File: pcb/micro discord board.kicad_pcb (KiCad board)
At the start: 2 copper layers, 71.4 x 57.2 mm, 9 parts, among them SW1 SW_Push, SW2 SW_Push, SW3 SW_Push, SW4 SW_Push, SW5 RotaryEncoder, U1 XIAO-RP2040-DIP

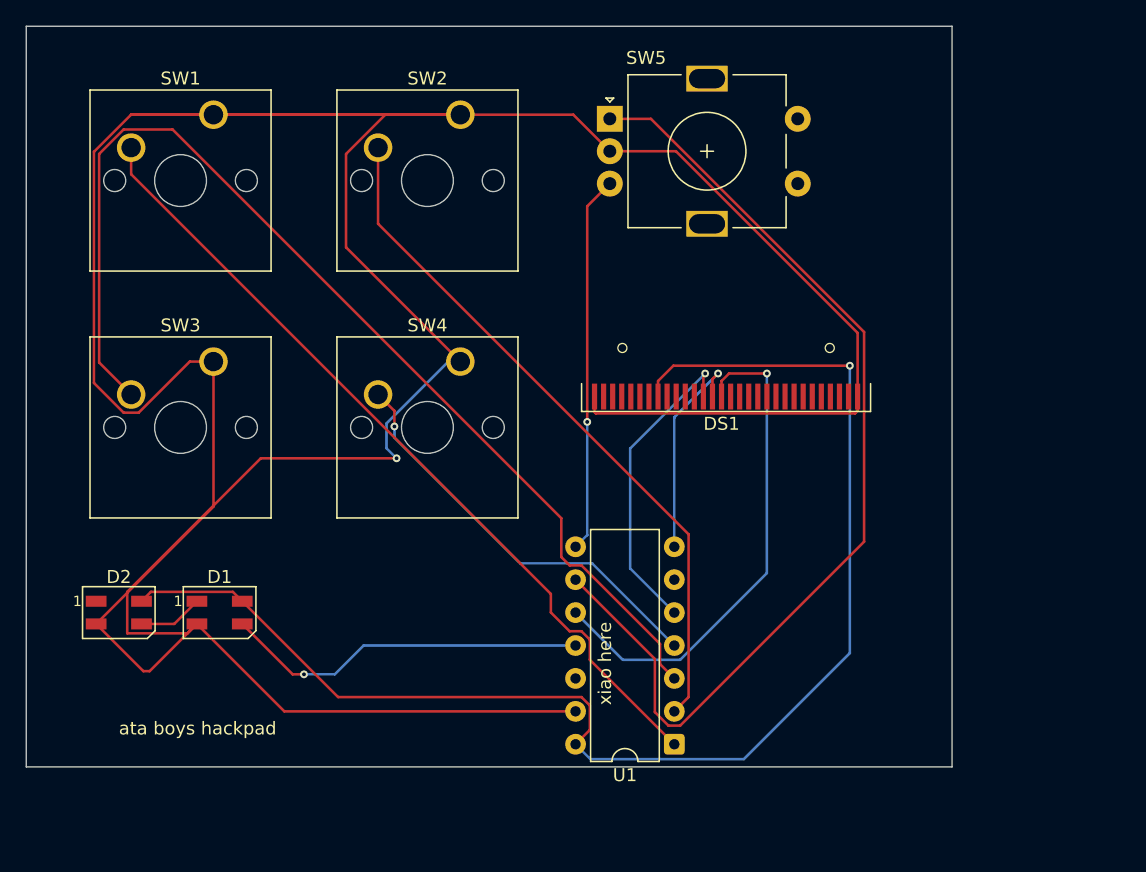
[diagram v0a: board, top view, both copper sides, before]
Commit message: Add files via upload
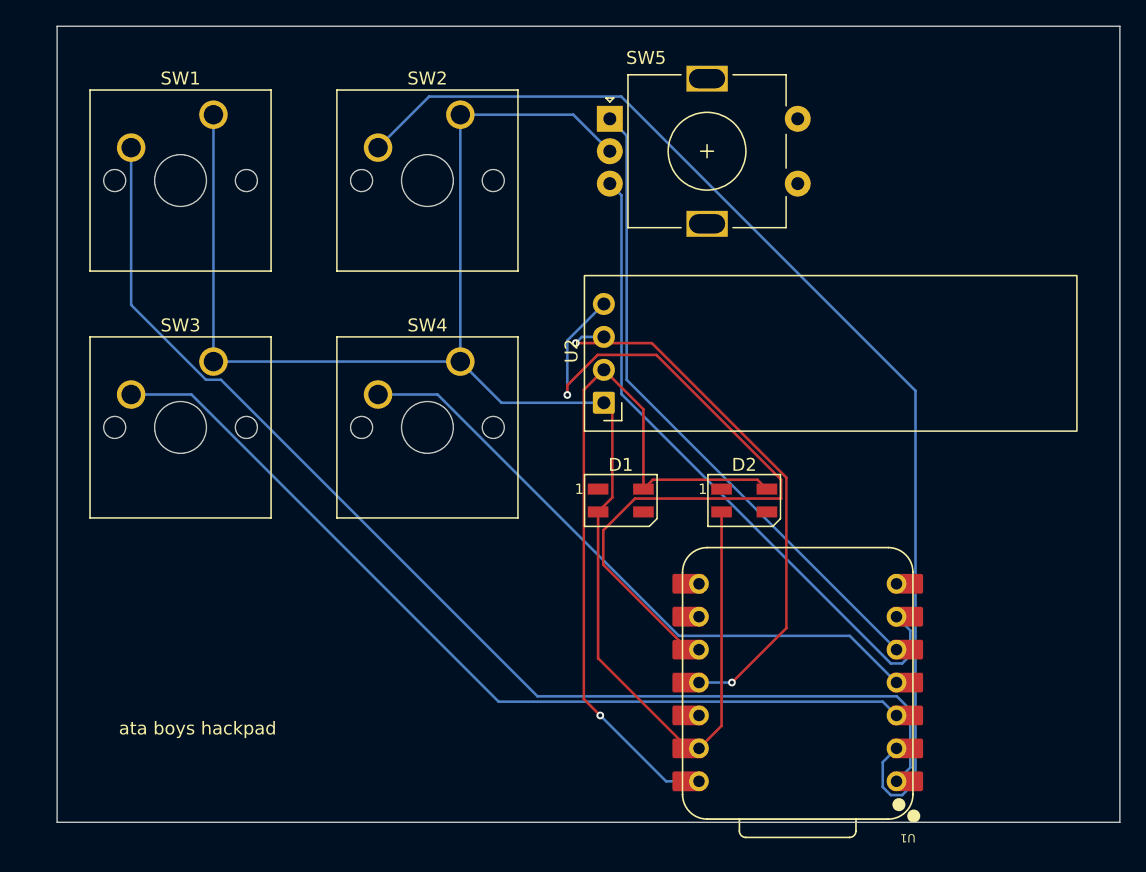
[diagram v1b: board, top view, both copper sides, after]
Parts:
- removed DS1: OLED-128O064D, Display:OLED-128O064D
- added U2: OLED_0.91_128x32, Hackclub Footprints:OLED_0.91_128x32, F.Cu at (118.4, 64.8)
- U1: value XIAO-RP2040-DIP -> XIAO-RP2040-SMD; footprint Package_DIP:DIP-14_W7.62mm -> Hackclub Footprints:XIAO-RP2040-DIP
- moved D2 49.0 mm to (129.2, 72.3)
- moved D1 32.1 mm to (119.7, 72.3)
- moved U1 10.6 mm to (133.3, 86.4)
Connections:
- SW5 pad A: Net-(U1-GPIO2/SCK) -> Net-(U1-GPIO6_D4_SDA)
- SW5 pad B: Net-(U1-GPIO1/RX) -> Net-(U1-GPIO7_D5_SCL)
- U1 pad 11: Net-(D1-DIN) -> Net-(U1-GPIO3_D10_MOSI)
- U1 pad 5: Net-(DS1-~{CS}) -> Net-(U1-GPIO6_D4_SDA)
- U1 pad 6: unconnected-(U1-GPIO7/SCL-Pad6) -> Net-(U1-GPIO7_D5_SCL)
- U1 pad 7: Net-(DS1-~{RES}) -> unconnected-(U1-GPIO0_D6_TX-Pad7)
- U1 pad 8: Net-(U1-GPIO1/RX) -> Net-(D1-DIN)
- U1 pad 9: Net-(U1-GPIO2/SCK) -> unconnected-(U1-GPIO2_D8_SCK-Pad9)
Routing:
- net GND: track 290.9 -> 131.5 mm, vias 1 -> 0
- net Net-(U1-GPIO2/SCK): track 77.8 -> 0.00 mm
- net Net-(U1-GPIO7_D5_SCL): track 0.00 -> 51.2 mm
- net Net-(U1-GPIO6_D4_SDA): track 0.00 -> 50.1 mm
- net +5V: track 105.7 -> 58.2 mm
- net Net-(U1-GPIO3_D10_MOSI): track 0.00 -> 43.0 mm, vias 0 -> 2
- net Net-(U1-GPIO27_A1_D1): track 53.9 -> 89.3 mm
- net Net-(U1-GPIO1/RX): track 29.1 -> 0.00 mm, vias 1 -> 0
- net Net-(D1-DIN): track 28.8 -> 0.00 mm, vias 1 -> 0
- net Net-(U1-GPIO26_A0_D0): track 63.9 -> 91.2 mm
- net Net-(DS1-~{CS}): track 24.8 -> 0.00 mm, vias 1 -> 0
- net Net-(U1-GPIO4_D9_MISO): track 39.4 -> 58.5 mm
- net Net-(U1-GPIO29_A3_D3): track 32.1 -> 49.2 mm, vias 1 -> 0
- net Net-(DS1-~{RES}): track 16.7 -> 0.00 mm, vias 1 -> 0
- net Net-(U1-GPIO28_A2_D2): track 85.0 -> 69.3 mm
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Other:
- board size 71.4 x 57.2 mm -> 82 x 61.4 mm
- board text removed: "xiao here"
